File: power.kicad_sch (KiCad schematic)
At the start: 43 parts, among them J14 Battery, J14 Main_Input_Jack, Q7 SI2301, SW3 SW, SW4 SW_SPST, U1 LM7805_TO220, U4 TP4056

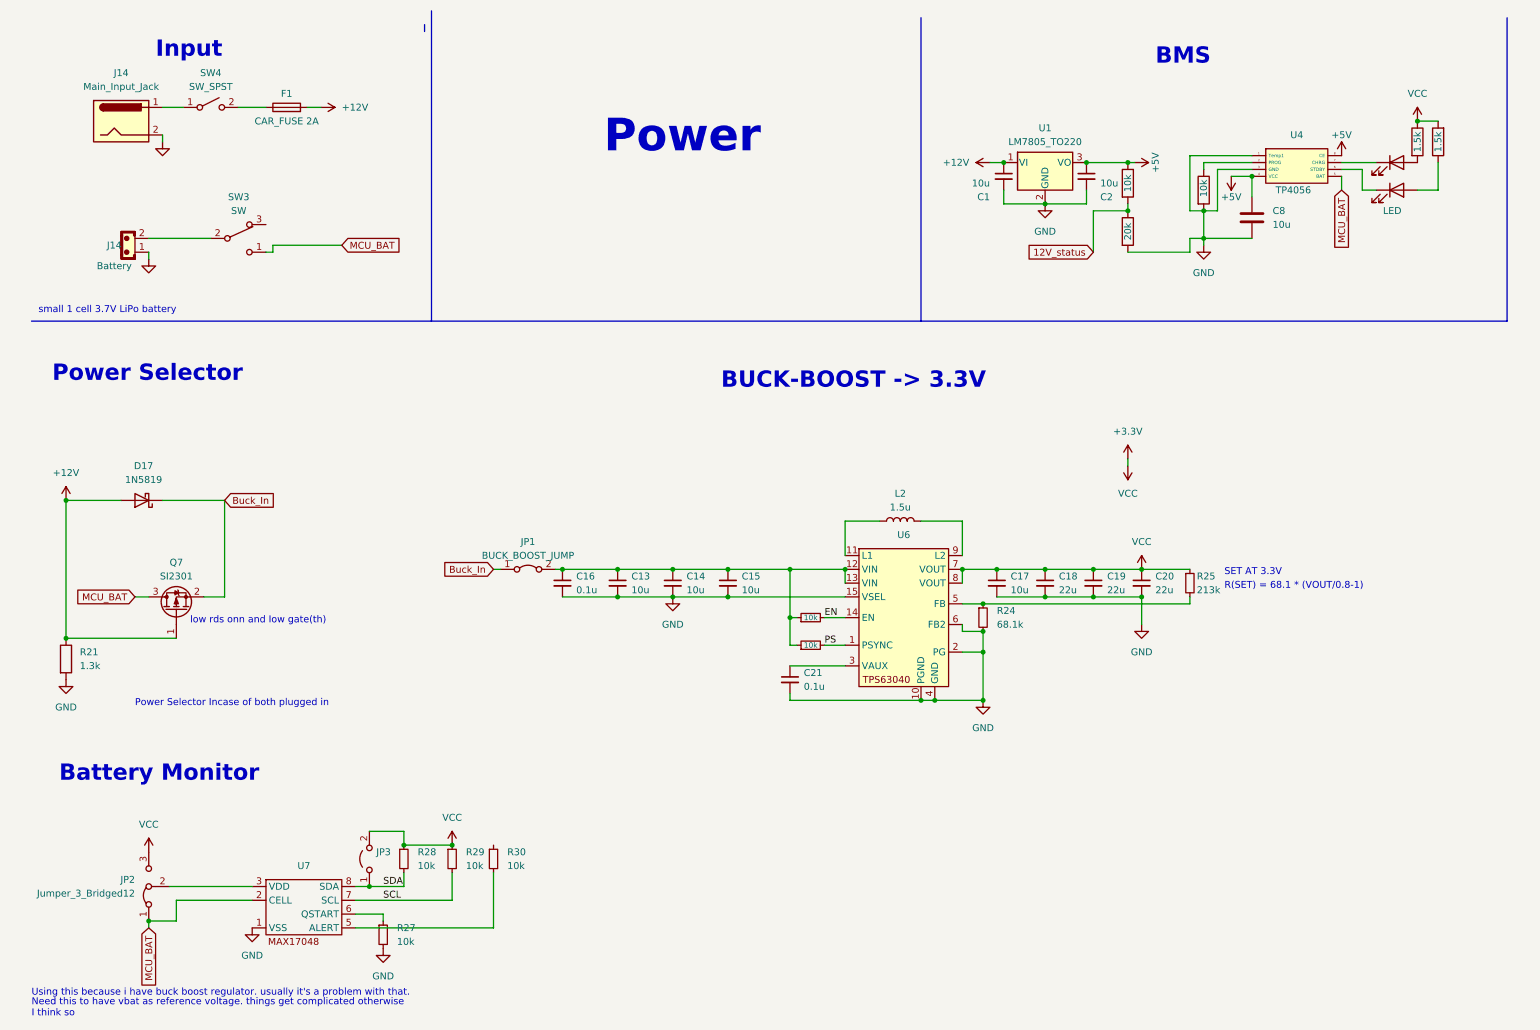
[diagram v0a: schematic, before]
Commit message: Schematic Completed
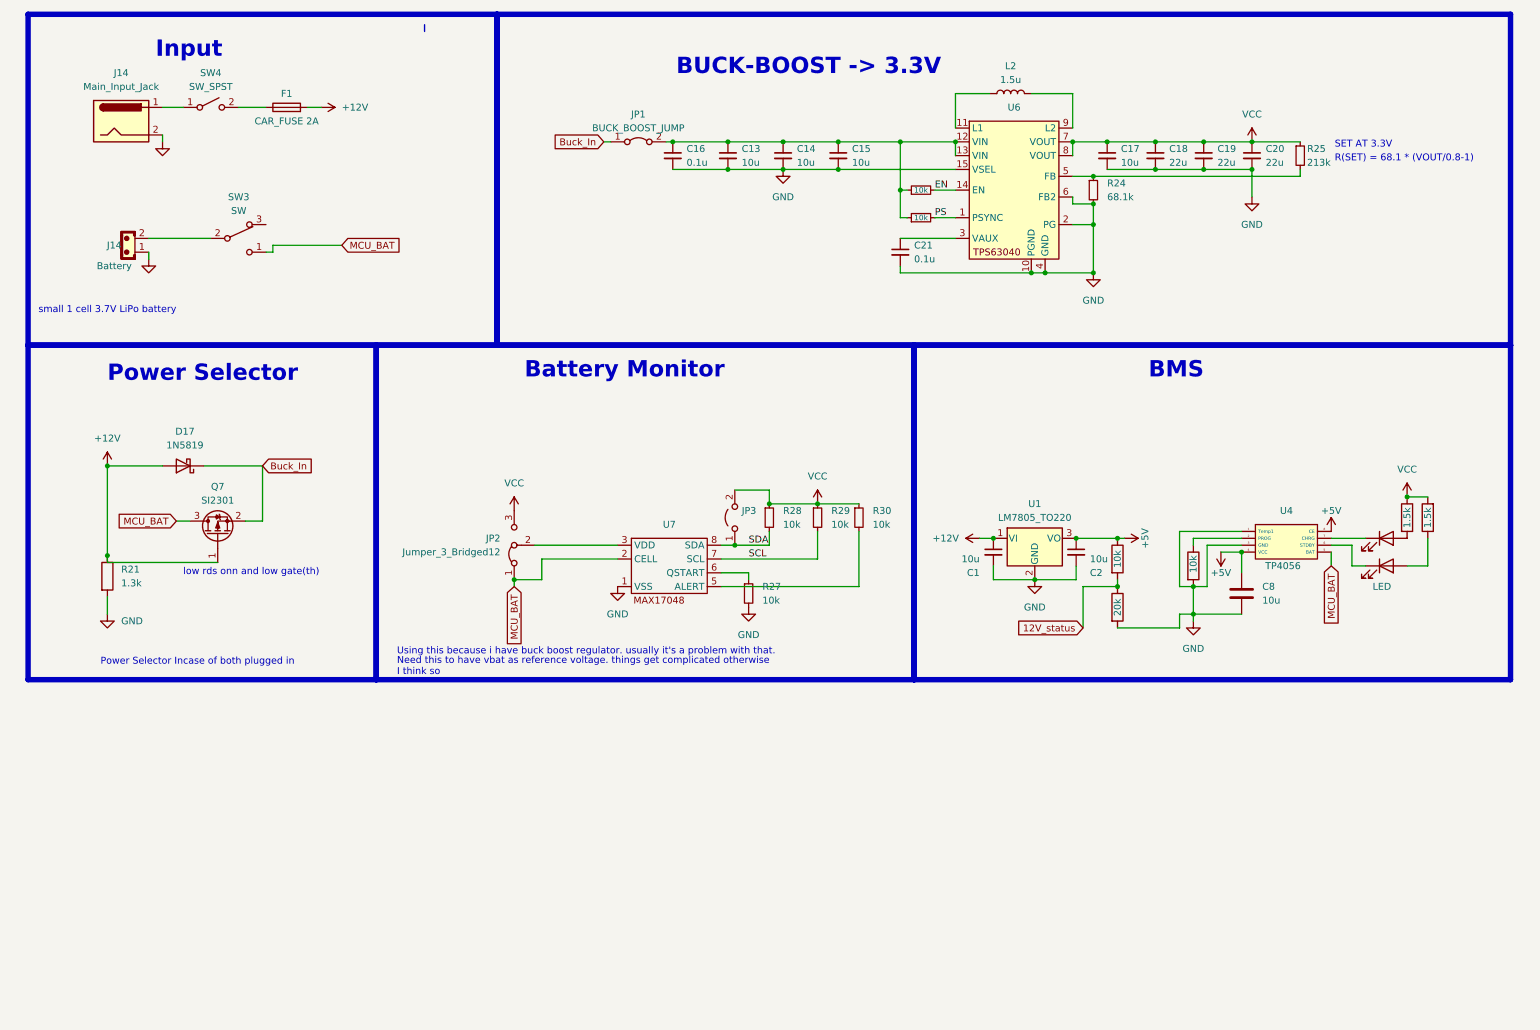
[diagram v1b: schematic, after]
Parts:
- removed R18: 20k, symbol Device:R
- removed R18: 1.5k, symbol Device:R
- removed R18: 10k, symbol Device:R
- added R18: 10k, symbol Device:R
- added R18: 20k, symbol Device:R
- added R18: 1.5k, symbol Device:R
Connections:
- net +3.3V is gone; now on net VCC: C17.1, C18.1, C19.1, C20.1, JP2.3 (B), JP3.2 (B), R17.2, R25.1, R28.1, R29.1, U6.7 (VOUT), U6.8 (VOUT)
- net +5V: now also R18.1
- net 12V_status: now also R18.1, R18.2
- net GND: now also R18.2
- net VCC: now reaches R30.1
- net VCC: now also R18.1
- net at D15.2 (A): now also R18.2
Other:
- note removed: "Power"
- moved on the sheet: C13, C14, C15, C16, C17, C18, C19, C20, C21, D17, JP1, JP2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
